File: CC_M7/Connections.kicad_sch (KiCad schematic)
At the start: 12 parts, among them J1 Conn_01x04_Pin, J10 Conn_01x04_Pin, J11 USB_B_Micro, J12 Conn_01x04_Pin, J3 Conn_01x03_Pin, J4 Conn_01x03_Pin, J5 Conn_01x03_Pin, J6 Conn_01x03_Pin, J7 Conn_01x03_Pin, J8 Conn_01x03_Pin

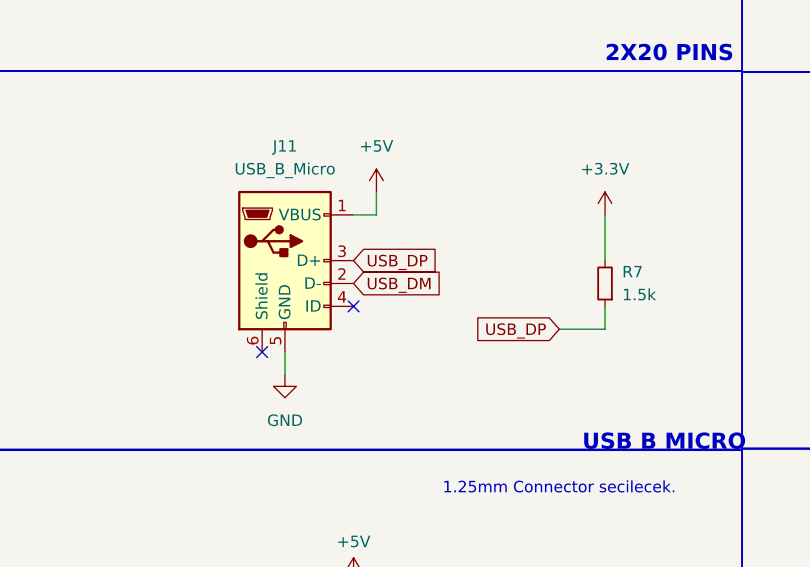
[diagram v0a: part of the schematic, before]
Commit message: last check
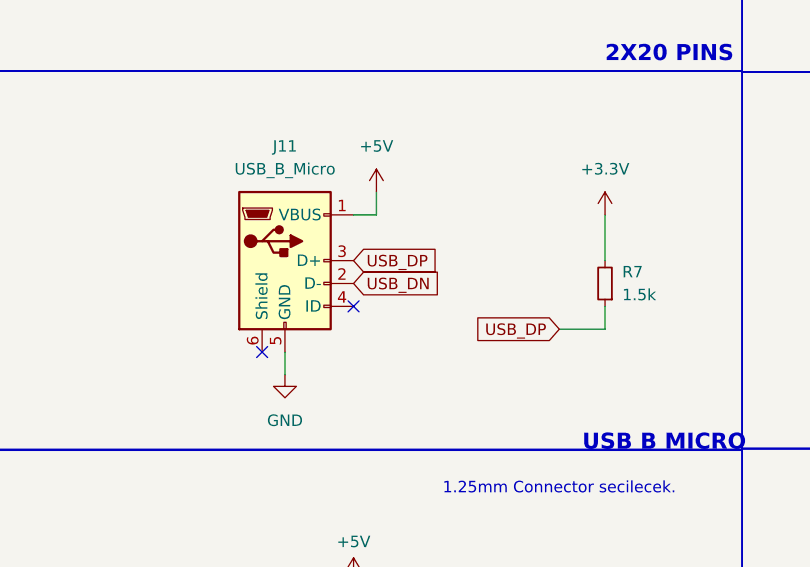
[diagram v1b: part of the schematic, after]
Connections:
- net USB_DM renamed USB_DN
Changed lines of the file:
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@@
 		)
 	)
-	(global_label "USB_DM"
+	(global_label "USB_DN"
 		(shape input)
 		(at 63.5 116.84 0)
@@
 		)
 		(property "Intersheetrefs" "${INTERSHEET_REFS}"
-			(at 73.9842 116.84 0)
+			(at 73.8633 116.84 0)
 			(effects
 				(font
